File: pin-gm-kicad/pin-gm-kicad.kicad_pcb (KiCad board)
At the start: 2 copper layers, 36 parts, among them U1 TL072, U2 LM358

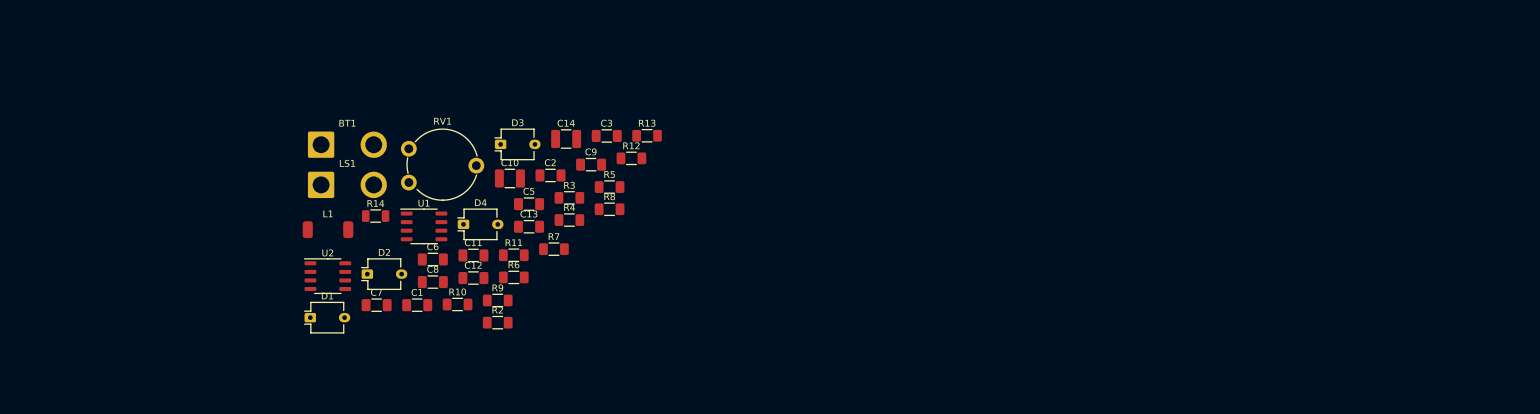
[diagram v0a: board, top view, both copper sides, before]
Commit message: kb semmi
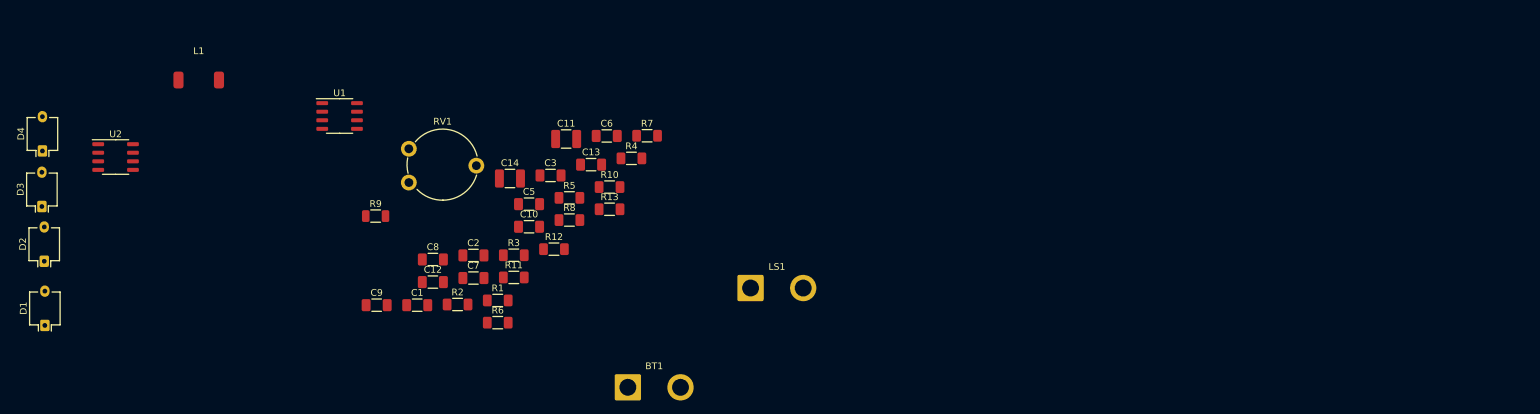
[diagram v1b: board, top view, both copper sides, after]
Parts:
- L1: value L -> 1m; footprint Inductor_SMD:L_Bourns_SRR0604_homemade -> Homemade:L_Bourns_SRR0604_homemade
- moved D2 69.8 mm to (144.1, 49.0), turned to 90 degrees
- moved LS1 65.4 mm to (248.7, 53.0)
- moved D1 63.8 mm to (144.2, 58.6), turned to 90 degrees
- moved BT1 57.9 mm to (230.5, 67.7)
- moved D3 49.3 mm to (143.7, 40.9), turned to 90 degrees
- moved U2 46.8 mm to (154.6, 33.6)
- moved D4 46.7 mm to (143.8, 32.7), turned to 90 degrees
- moved L1 29.3 mm to (167.0, 22.2)
- moved U1 23.8 mm to (187.8, 27.5)
- renumbered C13 to C10, C14 to C11, C8 to C12, C9 to C13, C10 to C14, C11 to C2, C2 to C3, C3 to C6, C12 to C7, C6 to C8, C7 to C9, D4 to D1, D3 to D2, D2 to D3, D1 to D4, R9 to R1, R5 to R10, R6 to R11, R7 to R12, R8 to R13, R10 to R2, R11 to R3, R12 to R4, R3 to R5, R2 to R6, R13 to R7, R4 to R8, R14 to R9, U2 to U1, U1 to U2

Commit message: kész vannak a footprintek
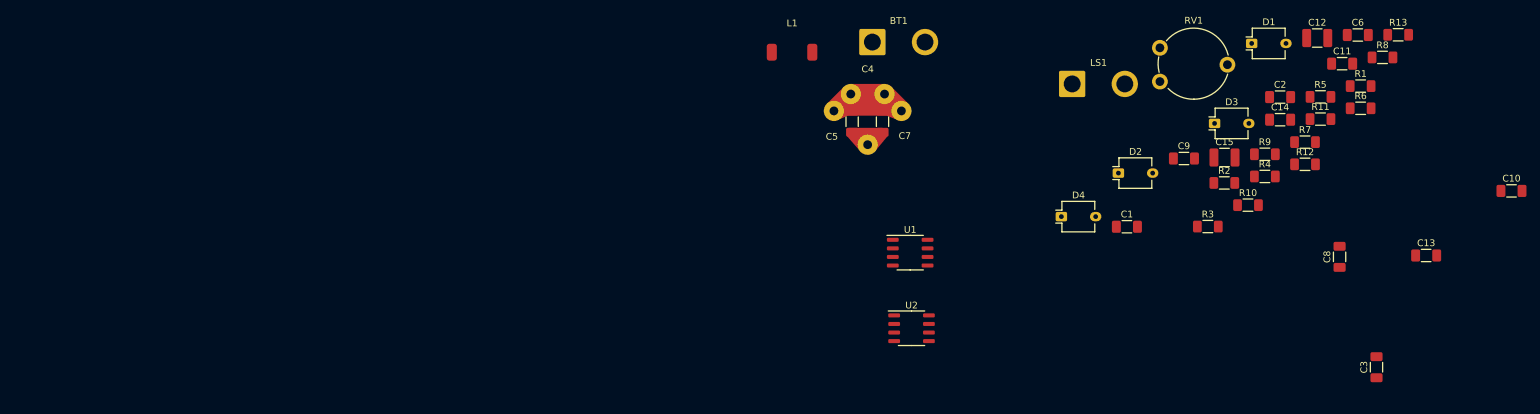
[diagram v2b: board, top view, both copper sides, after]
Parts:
- added C15: 47u, Capacitor_SMD:C_1210_3225Metric_Pad1.33x2.70mm_HandSolder, F.Cu at (318.9, 33.7)
- added C4: 10-40p, Homemade:C_trimmer_D10mm_homemade, F.Cu at (266.1, 26.8)
- C11, C14: value 47u -> 100n; footprint Capacitor_SMD:C_1210_3225Metric_Pad1.33x2.70mm_HandSolder -> Capacitor_SMD:C_1206_3216Metric_Pad1.33x1.80mm_HandSolder
- C12: value 10p -> 47u; footprint Capacitor_SMD:C_1206_3216Metric_Pad1.33x1.80mm_HandSolder -> Capacitor_SMD:C_1210_3225Metric_Pad1.33x2.70mm_HandSolder
- C13, C7, C8: value 100n -> 10p
- C6: value 10p -> 100n
- R9: footprint Resistor_SMD:R_1206_3216Metric -> Resistor_SMD:R_1206_3216Metric_Pad1.30x1.75mm_HandSolder
- moved D1 183.6 mm to (323.0, 16.8), turned to 0 degrees
- moved D3 174.2 mm to (317.5, 28.6), turned to 0 degrees
- moved D2 159.7 mm to (303.2, 36.0), turned to 0 degrees
- moved D4 151.3 mm to (294.8, 42.4), turned to 0 degrees
- moved C10 145.7 mm to (361.5, 38.6)
- moved C12 135.9 mm to (332.7, 16.0)
- moved C8 134.3 mm to (336.0, 48.4), turned to 90 degrees
- moved R9 132.1 mm to (324.9, 33.2)
- moved R1 131.7 mm to (339.1, 23.1)
- moved R6 131.7 mm to (339.1, 26.4)
- moved C3 125.6 mm to (341.5, 64.8), turned to 90 degrees
- moved C13 124.5 mm to (348.8, 48.2)
- moved R8 122.9 mm to (342.4, 18.9)
- moved R11 121.8 mm to (333.2, 28.0)
- moved C2 121.8 mm to (327.2, 24.7)
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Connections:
- net Net-(C3-Pad1) renamed /Diode_Cathode
- C10 pad 1: VCC -> Net-(C10-Pad1)
- C12 pad 1: Net-(C12-Pad1) -> VCC
- C12 pad 2: Net-(C12-Pad2) -> GND
- C13 pad 2: GND -> Net-(C13-Pad2)
- C14 pad 1: Net-(C13-Pad1) -> Net-(C14-Pad1)
- C6 pad 1: Net-(C3-Pad2) -> Net-(C6-Pad1)
- C7 pad 1: Net-(C7-Pad1) -> Net-(C3-Pad2)
- C7 pad 2: Net-(C7-Pad2) -> GND
- C8 pad 1: Net-(C6-Pad2) -> Net-(C3-Pad2)
- C9 pad 1: Net-(C9-Pad1) -> Net-(C8-Pad2)
- C9 pad 2: GND -> Net-(C9-Pad2)
- L1 pad 1: Net-(C13-Pad1) -> Net-(C14-Pad1)
- LS1 pad 1: Net-(C7-Pad2) -> Net-(C6-Pad2)
- R1 pad 1: Net-(C12-Pad2) -> Net-(C13-Pad2)
- R10 pad 1: Net-(C8-Pad2) -> Net-(C9-Pad2)
- R10 pad 2: Net-(C12-Pad1) -> Net-(C13-Pad1)
- R11 pad 1: Net-(C13-Pad1) -> Net-(C14-Pad1)
- R11 pad 2: Net-(C9-Pad1) -> Net-(C10-Pad1)
- R12 pad 1: Net-(C9-Pad1) -> Net-(C10-Pad1)
- R13 pad 1: Net-(C12-Pad1) -> Net-(C13-Pad1)
- R13 pad 2: Net-(C12-Pad2) -> Net-(C13-Pad2)
- R5 pad 1: Net-(C13-Pad1) -> Net-(C14-Pad1)
- R8 pad 2: Net-(C6-Pad2) -> Net-(R8-Pad2)
- R9 pad 2: Net-(C7-Pad1) -> Net-(C6-Pad1)
- U2 pad 1: Net-(C6-Pad2) -> Net-(R8-Pad2)
- U2 pad 5: Net-(C9-Pad1) -> Net-(C10-Pad1)
- U2 pad 6: Net-(C12-Pad1) -> Net-(C13-Pad1)
- U2 pad 7: Net-(C12-Pad2) -> Net-(C13-Pad2)
- U2 pad 8: Net-(C13-Pad1) -> Net-(C14-Pad1)
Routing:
- net Net-(C3-Pad2): track 0.00 -> 0.81 mm
